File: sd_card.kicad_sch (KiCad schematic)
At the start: 8 parts, among them J1 Micro_SD_Card

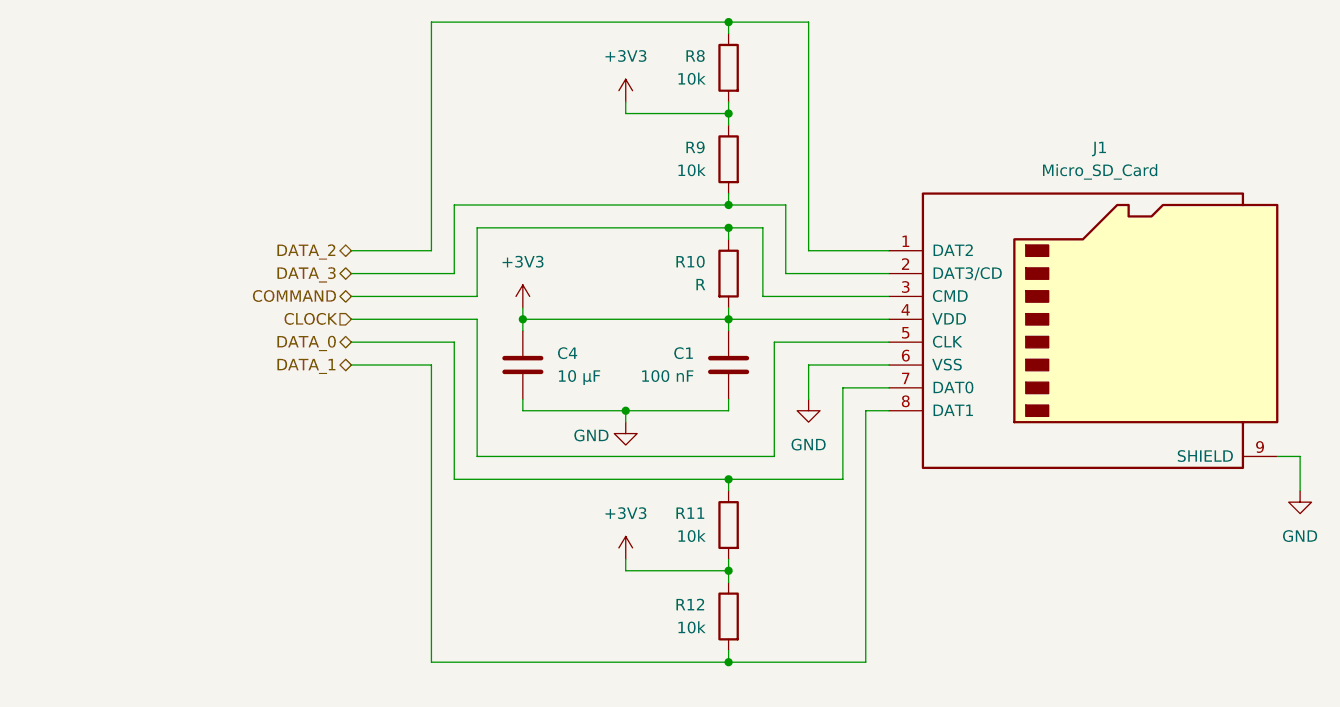
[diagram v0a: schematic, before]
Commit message: not adding this to source control months ago was one of the dumbest things i've ever done. and im not particularly risk-avers
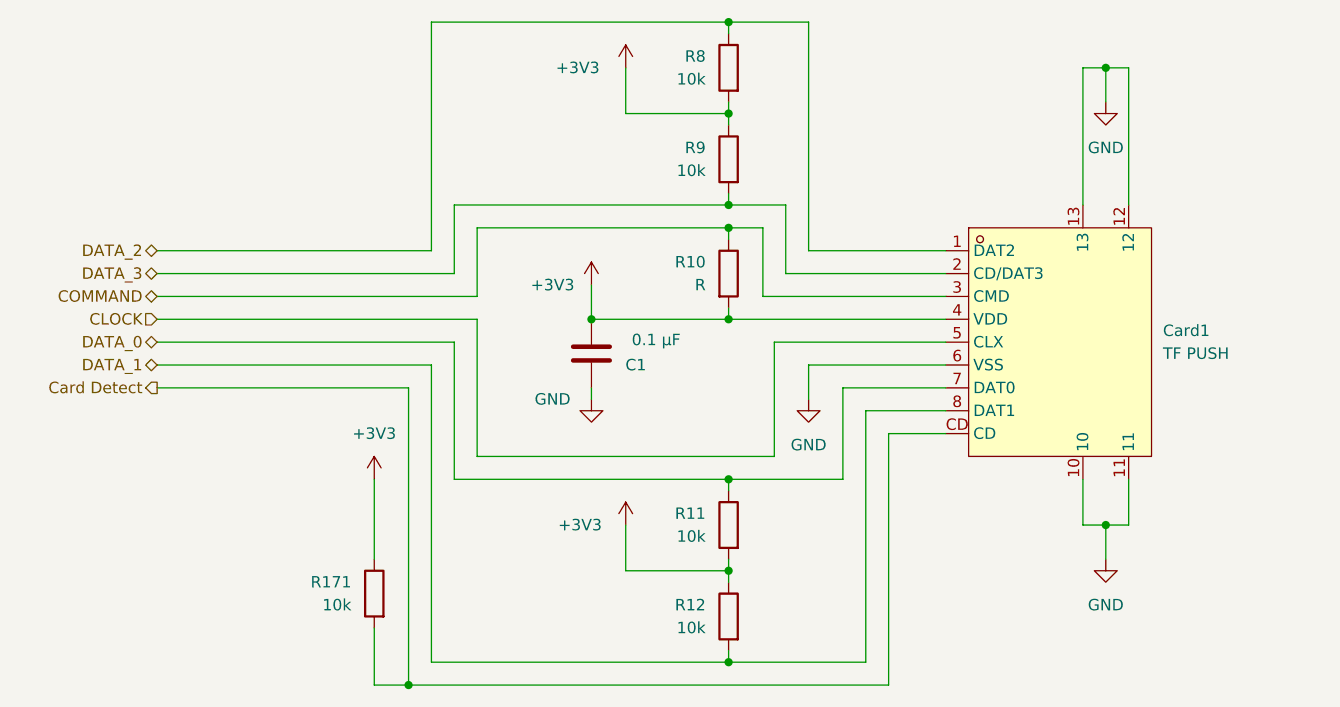
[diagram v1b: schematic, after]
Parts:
- removed C4: 10 µF, symbol Device:C
- removed J1: Micro_SD_Card, Connector_Card:microSD_HC_Wuerth_693072010801, symbol Connector:Micro_SD_Card
- added Card1: TF PUSH, easyeda2kicad:TF-SMD_TF-PUSH, symbol easyeda2kicad:TFPUSH
- added R171: 10k, symbol Device:R
- C1: value 100 nF -> 0.1 µF; footprint (none) -> easyeda2kicad:C0402; LCSC part number (none) -> C60474; Supplier (none) -> www.lcsc.com
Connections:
- net +3V3: now also Card1.4 (VDD), R171.1
- net CLOCK: now also Card1.5 (CLX)
- net COMMAND: now also Card1.3 (CMD)
- net DATA_0: now also Card1.7 (DAT0)
- net DATA_1: now also Card1.8 (DAT1)
- net DATA_2: now also Card1.1 (DAT2)
- net DATA_3: now also Card1.2 (CD/DAT3)
- net GND: now also Card1.10, Card1.11, Card1.12, Card1.13, Card1.6 (VSS)
- new net Card Detect: Card1.CD, R171.2
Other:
- moved on the sheet: C1
